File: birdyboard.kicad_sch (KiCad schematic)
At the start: 52 parts, among them J1 JST_3pin, J10 Conn_02x20_Odd_Even, J11 JST-PH StepMotor Conn, J12 TBP02R2-381-04BE, J13 Screw_Terminal_01x02, J14 Screw_Terminal_01x02, J15 Screw_Terminal_01x02, J16 JST-PH StepMotor Conn, J17 TBP02R2-381-04BE, J18 JST-PH StepMotor Conn, J19 TBP02R2-381-04BE, J2 JST_3pin, J20 JST-PH StepMotor Conn, J21 JST-PH UART Conn, J22 TBP02R2-381-04BE, J23 Conn_01x10, J24 AS5047_Adapter_Board_Connector, J25 AS5047_Adapter_Board_Connector, J26 AS5047_Adapter_Board_Connector, J27 AS5047_Adapter_Board_Connector, J4 JST_3pin, J5 JST_3pin, J6 JST_3pin, J7 JST_3pin, J8 JST_3pin, J9 JST_3pin, U1 TMC2209_SILENTSTEPSTICK, U2 TMC2209_SILENTSTEPSTICK, U3 Pico, U4 TMC2209_SILENTSTEPSTICK, U5 TMC2209_SILENTSTEPSTICK, U6 SN74CBT3253 MUX/DEMUX, U7 AZ1117CH-3_3TRG1, U8 K7805-3AR3

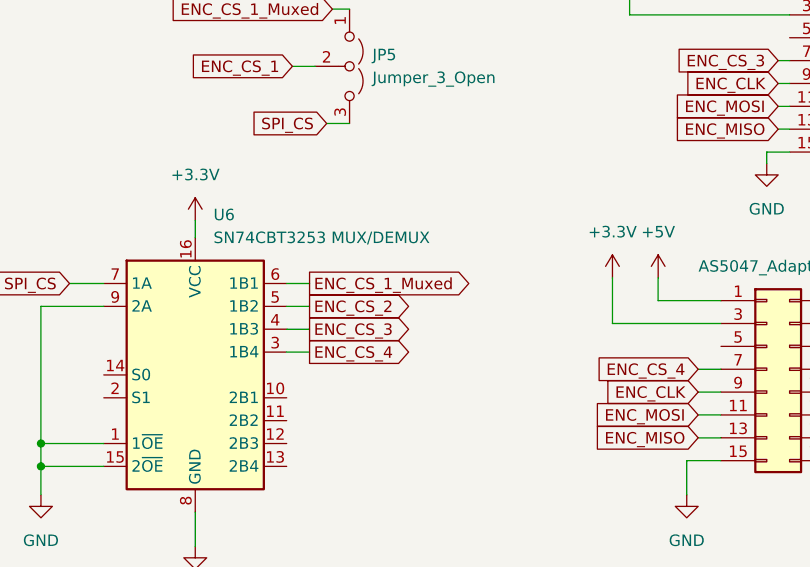
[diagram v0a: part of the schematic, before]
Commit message: lay out some routes - place last components
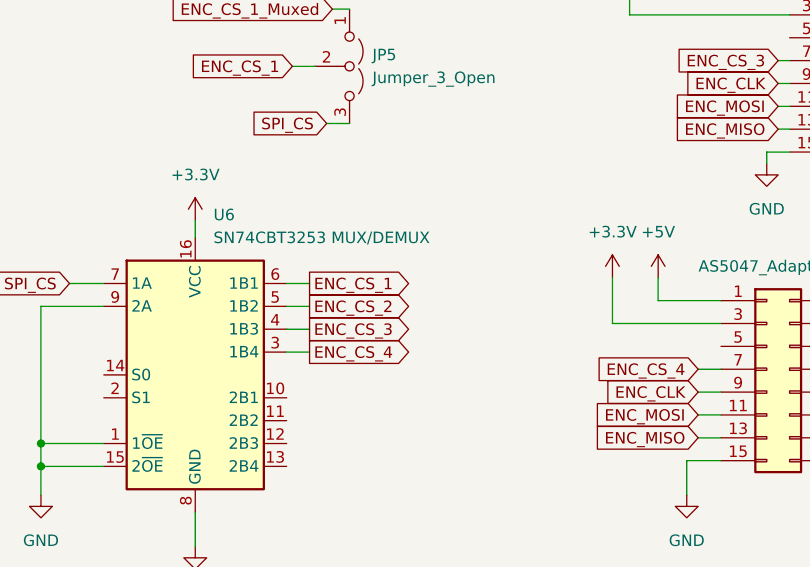
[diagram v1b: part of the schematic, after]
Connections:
- net ENC_CS_1: now also U6.6 (1B1)
- net ENC_CS_1_Muxed: no longer U6.6 (1B1)
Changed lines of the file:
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@@
     )
   )
-  (global_label "ENC_CS_1_Muxed" (shape output) (at 207.01 132.715 0) (fields_autoplaced)
+  (global_label "ENC_CS_1" (shape output) (at 207.01 132.715 0) (fields_autoplaced)
     (effects (font (size 1.27 1.27)) (justify left))
-    (property "Intersheet References" "${INTERSHEET_REFS}" (id 0) (at 225.6307 132.6356 0)
+    (property "Intersheet References" "${INTERSHEET_REFS}" (id 0) (at 218.7969 132.6356 0)
       (effects (font (size 1.27 1.27)) (justify left) hide)
     )
